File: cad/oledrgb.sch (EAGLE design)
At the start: 17 parts, among them U1 FAN5331SX

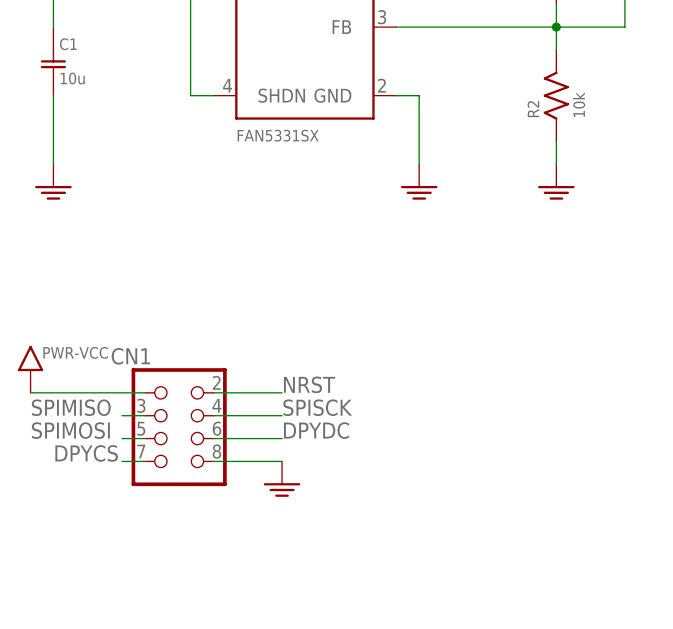
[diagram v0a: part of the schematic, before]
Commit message: embiggen connector
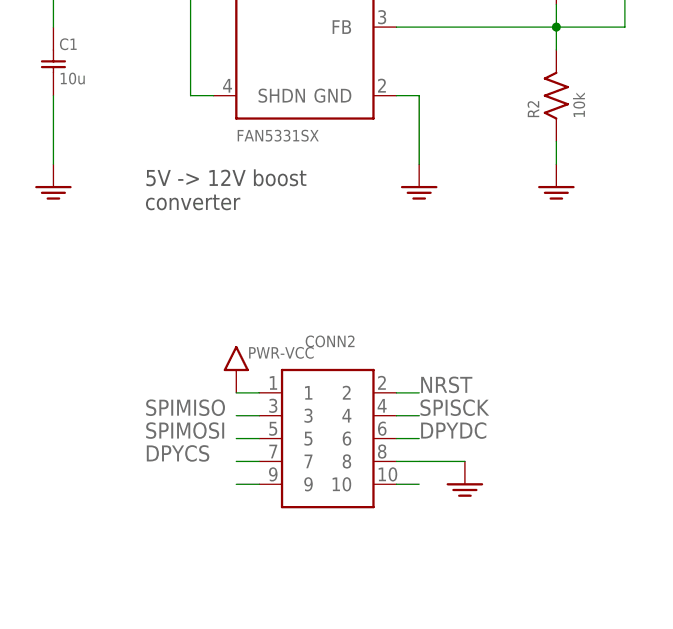
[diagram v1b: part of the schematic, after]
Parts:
- removed CN1: (no value), jaw:HEADER-2X4
- added CONN2: HEADER-5X2-PTH, jaw:HEADER-5X2-PTH
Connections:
- new net N$19: CONN2.10
- new net N$4: CONN2.9
- net DPYCS: now also CONN2.7; no longer CN1.P$7
- net DPYDC: now also CONN2.6; no longer CN1.P$6
- net GND: now also CONN2.8; no longer CN1.P$8
- net NRST: now also CONN2.2; no longer CN1.P$2
- net SPIMISO: now also CONN2.3; no longer CN1.P$3
- net SPIMOSI: now also CONN2.5; no longer CN1.P$5
- net SPISCK: now also CONN2.4; no longer CN1.P$4
- net VCC: now also CONN2.1; no longer CN1.P$1
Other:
- note added: "5V -> 12V boost converter"
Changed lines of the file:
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@@
 <parts>
 <part name="CONN1" library="jaw" deviceset="HEADER-22X1" device="-SMD8"/>
-<part name="CN1" library="jaw" deviceset="HEADER-2X4" device=""/>
-<part name="GND24" library="jaw" deviceset="PWR-GND" device=""/>
-<part name="VCC20" library="jaw" deviceset="PWR-VCC" device=""/>
 <part name="U1" library="microbuilder" deviceset="FAN5331" device="" value="FAN5331SX"/>
 <part name="GND1" library="jaw" deviceset="PWR-GND" device=""/>
@@
 <part name="U$3" library="adafruit" deviceset="FIDUCIAL" device=""/>
 <part name="LOGO1" library="Sparkfun-Aesthetics" deviceset="OSHW-LOGO" device="S"/>
+<part name="CONN2" library="jaw" deviceset="HEADER-5X2" device="-PTH"/>
+<part name="VCC2" library="jaw" deviceset="PWR-VCC" device=""/>
+<part name="GND7" library="jaw" deviceset="PWR-GND" device=""/>
 </parts>
 <sheets>
@@
 <text x="25.4" y="101.6" size="2.54" layer="97">crystalfontz RGB OLED 96x64
 ssd1332 based</text>
+<text x="33.02" y="48.26" size="1.778" layer="97">5V -&gt; 12V boost
+converter</text>
 </plain>
 <instances>
 <instance part="CONN1" gate="G$1" x="147.32" y="58.42"/>
-<instance part="CN1" gate="A" x="35.56" y="22.86"/>
-<instance part="GND24" gate="G$1" x="48.26" y="17.78"/>
-<instance part="VCC20" gate="G$1" x="20.32" y="30.48"/>
 <instance part="U1" gate="G$1" x="50.8" y="68.58"/>
 <instance part="GND1" gate="G$1" x="22.86" y="50.8"/>
@@
 <instance part="U$3" gate="G$1" x="132.08" y="10.16"/>
 <instance part="LOGO1" gate="G$1" x="149.86" y="12.7"/>
+<instance part="CONN2" gate="G$1" x="53.34" y="17.78"/>
+<instance part="VCC2" gate="G$1" x="43.18" y="30.48"/>
+<instance part="GND7" gate="G$1" x="68.58" y="17.78"/>
 </instances>
 <busses>
@@
 <nets>
 <net name="GND" class="0">
-<segment>
-<pinref part="CN1" gate="A" pin="P$8"/>
-<pinref part="GND24" gate="G$1" pin="GND"/>
-<wire x1="48.26" y1="20.32" x2="40.64" y2="20.32" width="0.1524" layer="91"/>
-</segment>
 <segment>
 <wire x1="22.86" y1="60.96" x2="22.86" y2="53.34" width="0.1524" layer="91"/>
@@
 <label x="129.54" y="35.56" size="1.27" layer="95"/>
 </segment>
+<segment>
+<pinref part="CONN2" gate="G$1" pin="8"/>
+<wire x1="60.96" y1="20.32" x2="63.5" y2="20.32" width="0.1524" layer="91"/>
+<pinref part="GND7" gate="G$1" pin="GND"/>
+<wire x1="63.5" y1="20.32" x2="68.58" y2="20.32" width="0.1524" layer="91"/>
+</segment>
 </net>
 <net name="VCC" class="0">
-<segment>
-<pinref part="CN1" gate="A" pin="P$1"/>
-<pinref part="VCC20" gate="G$1" pin="VCC"/>
-<wire x1="20.32" y1="27.94" x2="33.02" y2="27.94" width="0.1524" layer="91"/>
-</segment>
 <segment>
 <wire x1="22.86" y1="76.2" x2="22.86" y2="68.58" width="0.1524" layer="91"/>
@@
 <label x="129.54" y="81.28" size="1.27" layer="95"/>
 </segment>
+<segment>
+<pinref part="CONN2" gate="G$1" pin="1"/>
+<wire x1="45.72" y1="27.94" x2="43.18" y2="27.94" width="0.1524" layer="91"/>
+<pinref part="VCC2" gate="G$1" pin="VCC"/>
+</segment>
 </net>
 <net name="NRST" class="0">
 <segment>
-<pinref part="CN1" gate="A" pin="P$2"/>
-<wire x1="40.64" y1="27.94" x2="48.26" y2="27.94" width="0.1524" layer="91"/>
-<label x="48.26" y="27.94" size="1.778" layer="95"/>
+<pinref part="CONN2" gate="G$1" pin="2"/>
+<wire x1="60.96" y1="27.94" x2="63.5" y2="27.94" width="0.1524" layer="91"/>
+<label x="63.5" y="27.94" size="1.778" layer="95"/>
 </segment>
 <segment>
@@
 <net name="DPYDC" class="0">
 <segment>
-<pinref part="CN1" gate="A" pin="P$6"/>
-<wire x1="40.64" y1="22.86" x2="48.26" y2="22.86" width="0.1524" layer="91"/>
-<label x="48.26" y="22.86" size="1.778" layer="95"/>
-</segment>
-<segment>
 <pinref part="CONN1" gate="G$1" pin="15"/>
 <wire x1="147.32" y1="48.26" x2="137.16" y2="48.26" width="0.1524" layer="91"/>
 <label x="129.54" y="48.26" size="1.27" layer="95"/>
 </segment>
+<segment>
+<pinref part="CONN2" gate="G$1" pin="6"/>
+<wire x1="60.96" y1="22.86" x2="63.5" y2="22.86" width="0.1524" layer="91"/>
+<label x="63.5" y="22.86" size="1.778" layer="95"/>
+</segment>
 </net>
 <net name="SPISCK" class="0">
-<segment>
-<pinref part="CN1" gate="A" pin="P$4"/>
-<wire x1="40.64" y1="25.4" x2="48.26" y2="25.4" width="0.1524" layer="91"/>
-<label x="48.26" y="25.4" size="1.778" layer="95"/>
-</segment>
 <segment>
 <pinref part="CONN1" gate="G$1" pin="12"/>
@@
 <label x="129.54" y="55.88" size="1.27" layer="95"/>
 </segment>
+<segment>
+<pinref part="CONN2" gate="G$1" pin="4"/>
+<wire x1="60.96" y1="25.4" x2="63.5" y2="25.4" width="0.1524" layer="91"/>
+<label x="63.5" y="25.4" size="1.778" layer="95"/>
+</segment>
 </net>
 <net name="SPIMISO" class="0">
 <segment>
-<pinref part="CN1" gate="A" pin="P$3"/>
-<wire x1="33.02" y1="25.4" x2="30.48" y2="25.4" width="0.1524" layer="91"/>
-<label x="20.32" y="25.4" size="1.778" layer="95"/>
+<pinref part="CONN2" gate="G$1" pin="3"/>
+<wire x1="45.72" y1="25.4" x2="43.18" y2="25.4" width="0.1524" layer="91"/>
+<label x="33.02" y="25.4" size="1.778" layer="95"/>
 </segment>
 </net>
 <net name="SPIMOSI" class="0">
-<segment>
-<pinref part="CN1" gate="A" pin="P$5"/>
-<wire x1="33.02" y1="22.86" x2="30.48" y2="22.86" width="0.1524" layer="91"/>
-<label x="20.32" y="22.86" size="1.778" layer="95"/>
-</segment>
 <segment>
 <pinref part="CONN1" gate="G$1" pin="11"/>
@@
 <label x="129.54" y="58.42" size="1.27" layer="95"/>
 </segment>
+<segment>
+<pinref part="CONN2" gate="G$1" pin="5"/>
+<wire x1="45.72" y1="22.86" x2="43.18" y2="22.86" width="0.1524" layer="91"/>
+<label x="33.02" y="22.86" size="1.778" layer="95"/>
+</segment>
 </net>
 <net name="DPYCS" class="0">
-<segment>
-<pinref part="CN1" gate="A" pin="P$7"/>
-<wire x1="33.02" y1="20.32" x2="30.48" y2="20.32" width="0.1524" layer="91"/>
-<label x="22.86" y="20.32" size="1.778" layer="95"/>
-</segment>
 <segment>
 <pinref part="CONN1" gate="G$1" pin="17"/>
 <wire x1="147.32" y1="43.18" x2="137.16" y2="43.18" width="0.1524" layer="91"/>
 <label x="129.54" y="43.18" size="1.27" layer="95"/>
+</segment>
+<segment>
+<pinref part="CONN2" gate="G$1" pin="7"/>
+<wire x1="45.72" y1="20.32" x2="43.18" y2="20.32" width="0.1524" layer="91"/>
+<label x="33.02" y="20.32" size="1.778" layer="95"/>
 </segment>
 </net>
@@
 </segment>
 </net>
+<net name="N$4" class="0">
+<segment>
+<pinref part="CONN2" gate="G$1" pin="9"/>
+<wire x1="45.72" y1="17.78" x2="43.18" y2="17.78" width="0.1524" layer="91"/>
+</segment>
+</net>
+<net name="N$19" class="0">
+<segment>
+<pinref part="CONN2" gate="G$1" pin="10"/>
+<wire x1="60.96" y1="17.78" x2="63.5" y2="17.78" width="0.1524" layer="91"/>
+</segment>
+</net>
